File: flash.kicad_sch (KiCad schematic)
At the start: 1 part, among them U8 28F400

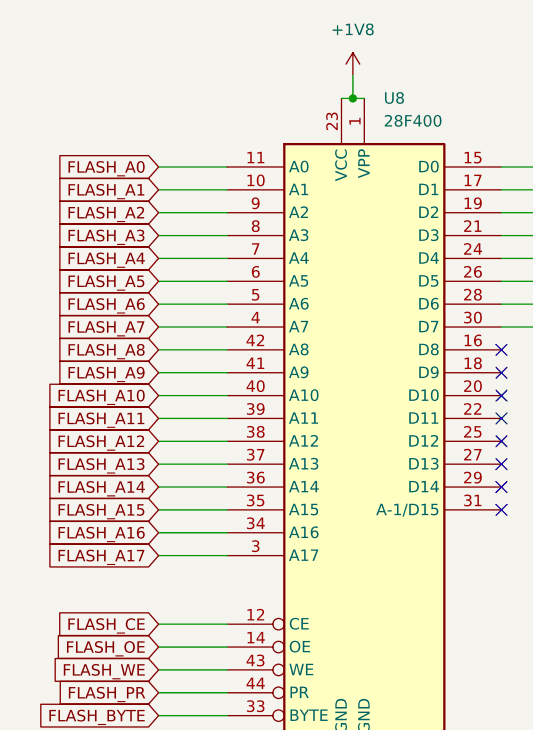
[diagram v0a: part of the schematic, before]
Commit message: morning
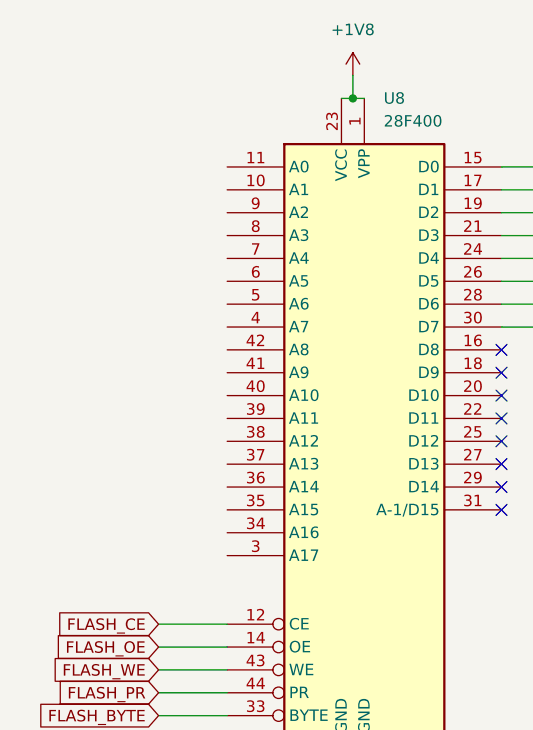
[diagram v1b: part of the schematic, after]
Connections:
- net FLASH_A0: no longer names the net of U8.11 (A0)
- net FLASH_A1: no longer names the net of U8.10 (A1)
- net FLASH_A10: no longer names the net of U8.40 (A10)
- net FLASH_A11: no longer names the net of U8.39 (A11)
- net FLASH_A12: no longer names the net of U8.38 (A12)
- net FLASH_A13: no longer names the net of U8.37 (A13)
- net FLASH_A14: no longer names the net of U8.36 (A14)
- net FLASH_A15: no longer names the net of U8.35 (A15)
- net FLASH_A16: no longer names the net of U8.34 (A16)
- net FLASH_A17: no longer names the net of U8.3 (A17)
- net FLASH_A2: no longer names the net of U8.9 (A2)
- net FLASH_A3: no longer names the net of U8.8 (A3)
- net FLASH_A4: no longer names the net of U8.7 (A4)
- net FLASH_A5: no longer names the net of U8.6 (A5)
- net FLASH_A6: no longer names the net of U8.5 (A6)
- net FLASH_A7: no longer names the net of U8.4 (A7)
- net FLASH_A8: no longer names the net of U8.42 (A8)
- net FLASH_A9: no longer names the net of U8.41 (A9)

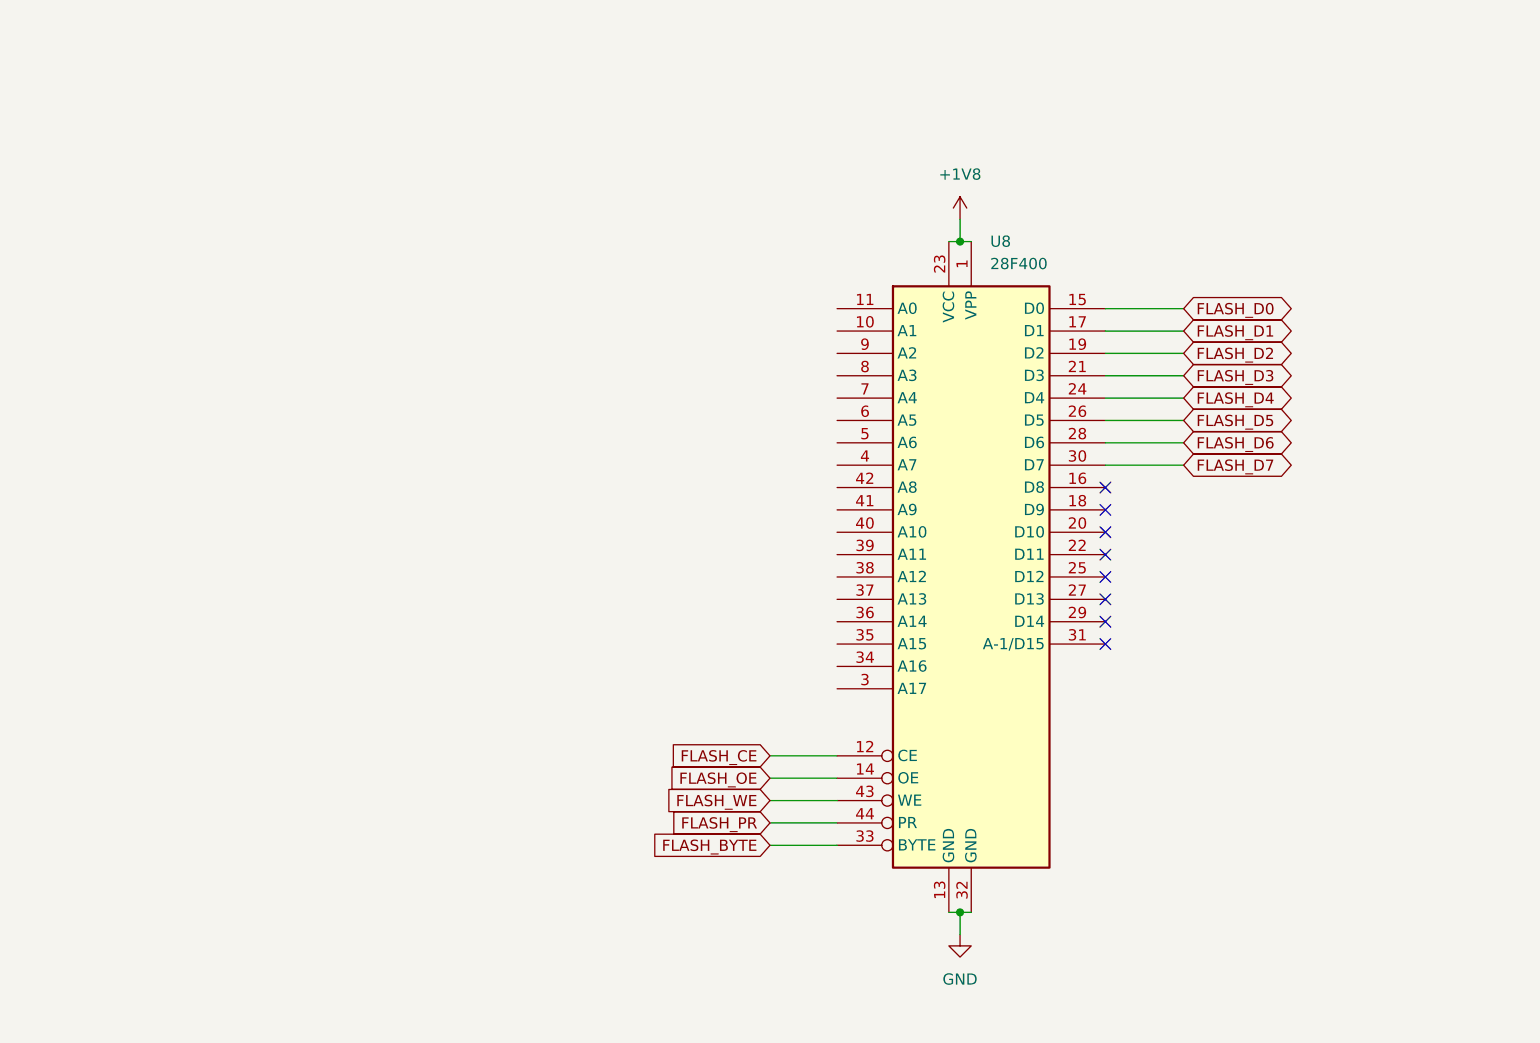
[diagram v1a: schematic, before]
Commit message: before caleb
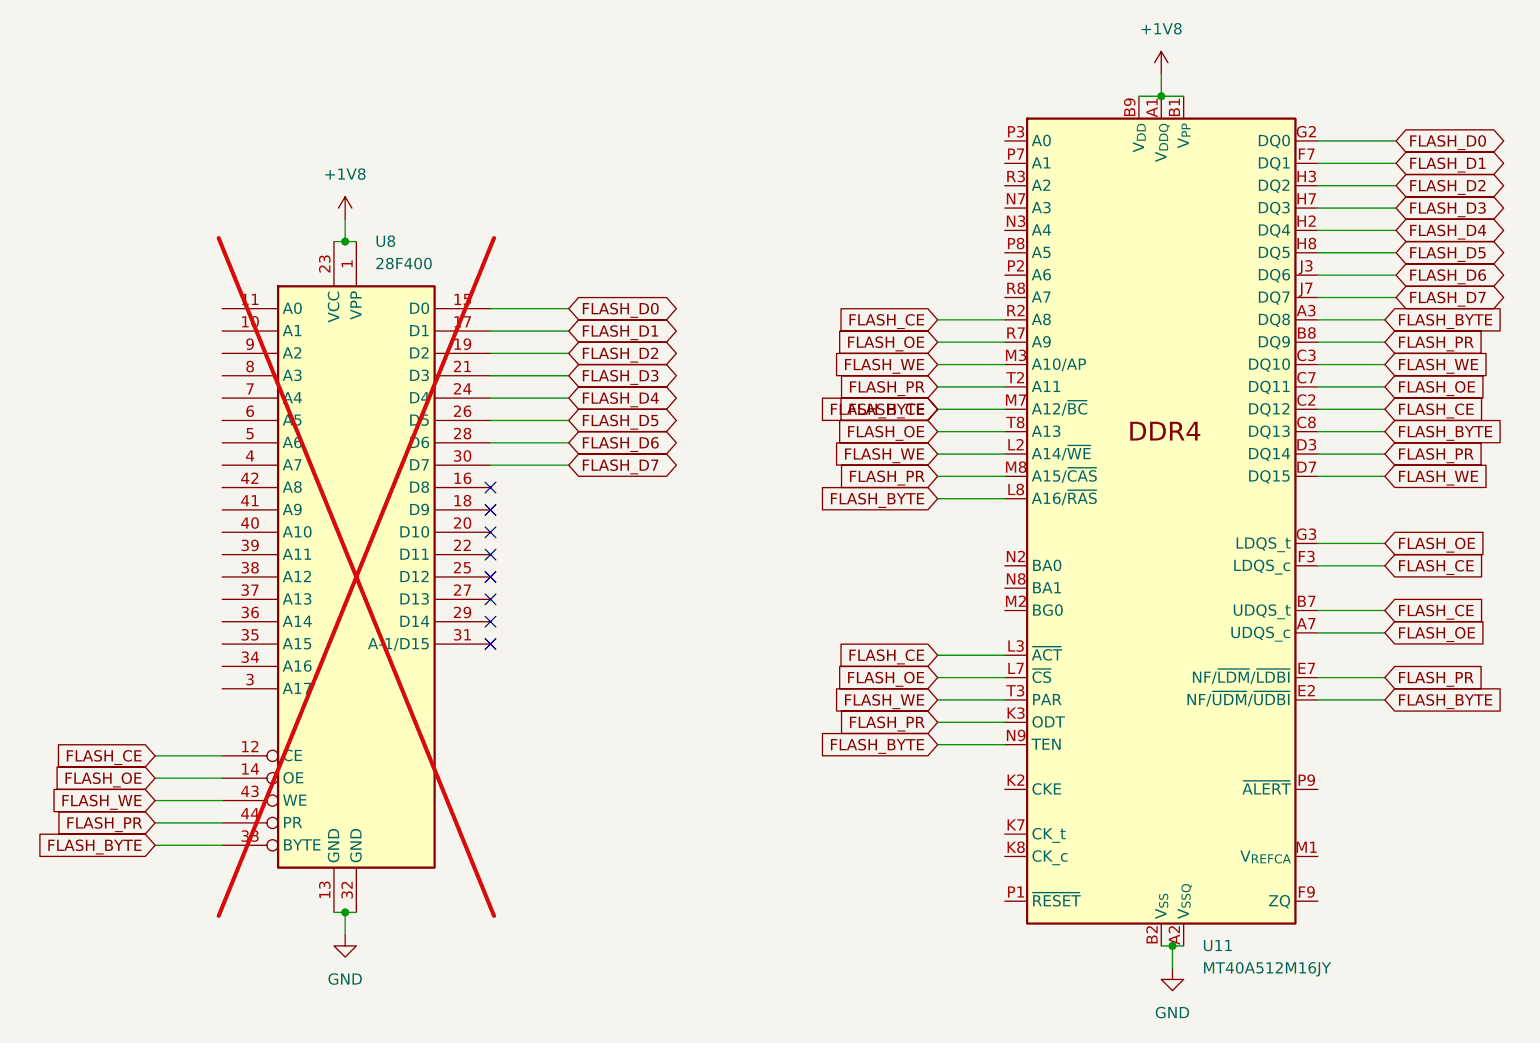
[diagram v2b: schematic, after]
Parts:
- added U11: MT40A512M16JY, Package_BGA:BGA-63_9x11mm_Layout10x12_P0.8mm, symbol Memory_RAM:MT40A512M16JY
- U8: now not fitted; now left out of the parts list
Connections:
- net FLASH_CE is gone; now on net FLASH_BYTE: U8.12 (CE)
- net +1V8: now also U11.A1 (V_{DDQ}), U11.A9 (V_{DDQ}), U11.B1 (V_{PP}), U11.B3 (V_{DD}), U11.B9 (V_{DD}), U11.C1 (V_{DDQ}), U11.D1 (V_{DD}), U11.D9 (V_{DDQ}), U11.F2 (V_{DDQ}), U11.F8 (V_{DDQ}), U11.G1 (V_{DDQ}), U11.G7 (V_{DD}), U11.G9 (V_{DDQ}), U11.J1 (V_{DD}), U11.J2 (V_{DDQ}), U11.J8 (V_{DDQ}), U11.J9 (V_{DD}), U11.L1 (V_{DD}), U11.L9 (V_{DD}), U11.R1 (V_{DD}), U11.R9 (V_{PP}), U11.T9 (V_{DD})
- net FLASH_BYTE: now also U11.A3 (DQ8), U11.B7 (UDQS_t), U11.C2 (DQ12), U11.C8 (DQ13), U11.E2 (NF/~{UDM}/~{UDBI}), U11.F3 (LDQS_c), U11.L3 (~{ACT}), U11.L8 (A16/~{RAS}), U11.M7 (A12/~{BC}), U11.N9 (TEN), U11.R2 (A8)
- net FLASH_D0: now also U11.G2 (DQ0)
- net FLASH_D1: now also U11.F7 (DQ1)
- net FLASH_D2: now also U11.H3 (DQ2)
- net FLASH_D3: now also U11.H7 (DQ3)
- net FLASH_D4: now also U11.H2 (DQ4)
- net FLASH_D5: now also U11.H8 (DQ5)
- net FLASH_D6: now also U11.J3 (DQ6)
- net FLASH_D7: now also U11.J7 (DQ7)
- net FLASH_OE: now also U11.A7 (UDQS_c), U11.C7 (DQ11), U11.G3 (LDQS_t), U11.L7 (~{CS}), U11.R7 (A9), U11.T8 (A13)
- net FLASH_PR: now also U11.B8 (DQ9), U11.D3 (DQ14), U11.E7 (NF/~{LDM}/~{LDBI}), U11.K3 (ODT), U11.M8 (A15/~{CAS}), U11.T2 (A11)
- net FLASH_WE: now also U11.C3 (DQ10), U11.D7 (DQ15), U11.L2 (A14/~{WE}), U11.M3 (A10/AP), U11.T3 (PAR)
- net GND: now also U11.A2 (V_{SSQ}), U11.A8 (V_{SSQ}), U11.B2 (V_{SS}), U11.C9 (V_{SSQ}), U11.D2 (V_{SSQ}), U11.D8 (V_{SSQ}), U11.E1 (V_{SS}), U11.E3 (V_{SSQ}), U11.E8 (V_{SSQ}), U11.E9 (V_{SS}), U11.F1 (V_{SSQ}), U11.G8 (V_{SS}), U11.H1 (V_{SSQ}), U11.H9 (V_{SSQ}), U11.K1 (V_{SS}), U11.K9 (V_{SS}), U11.M9 (V_{SS}), U11.N1 (V_{SS}), U11.T1 (V_{SS})

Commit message: after rough draft submission
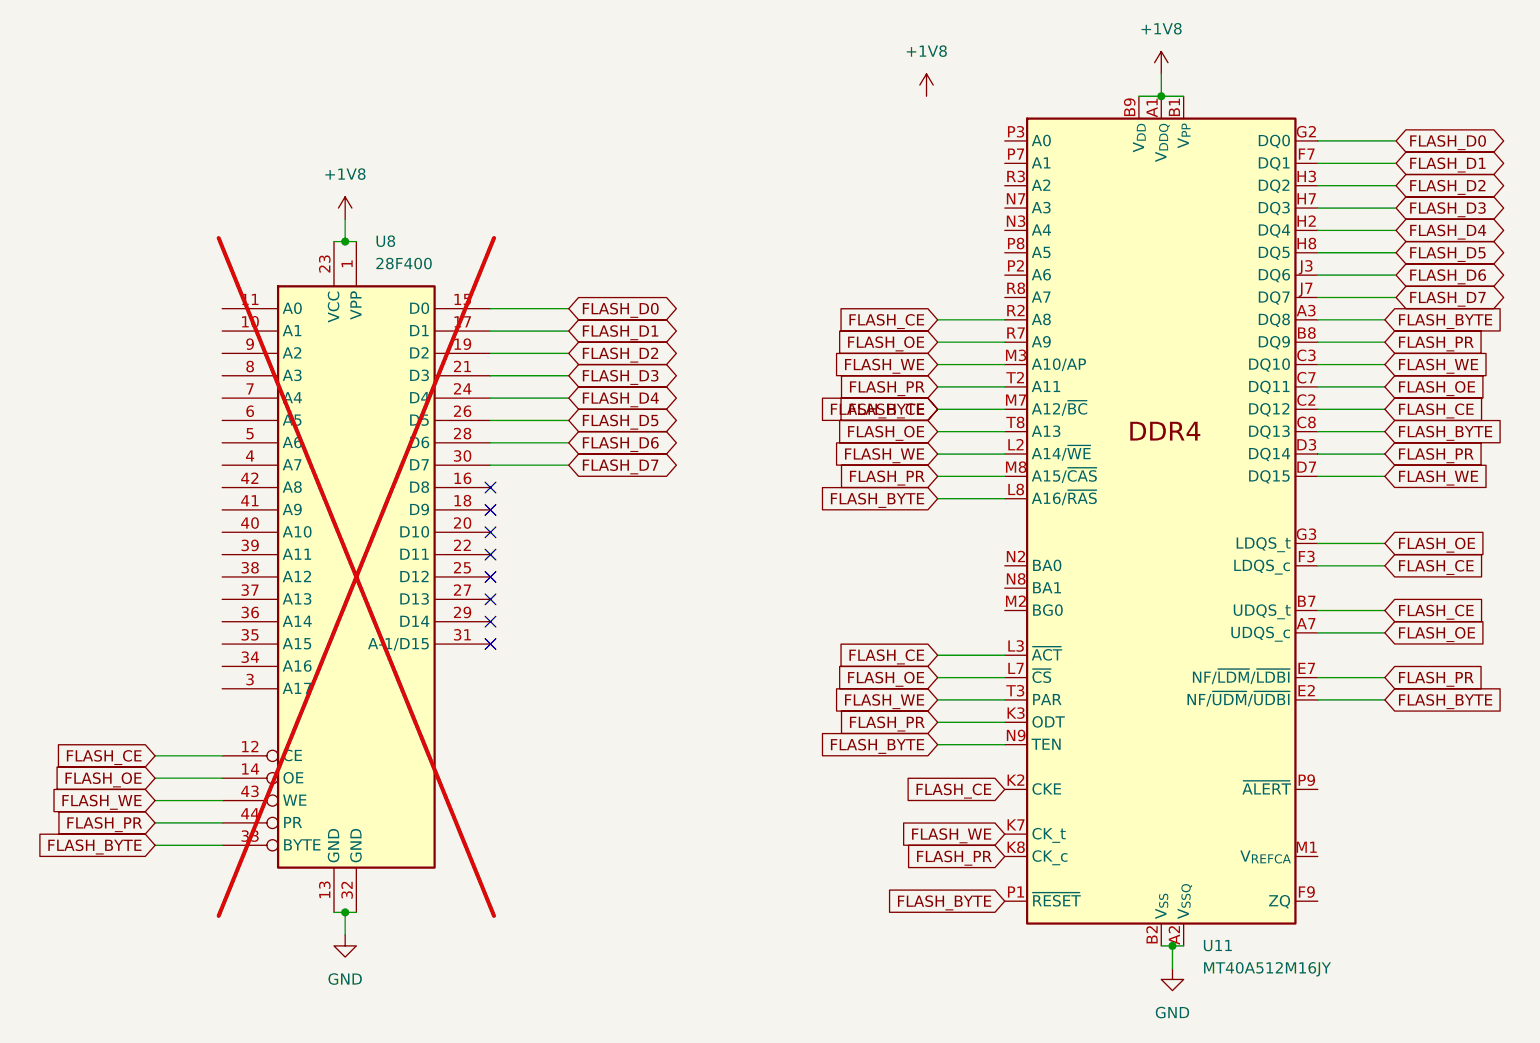
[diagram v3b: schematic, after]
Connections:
- net FLASH_BYTE: now also U11.K2 (CKE), U11.P1 (~{RESET})
- net FLASH_PR: now also U11.K8 (CK_c)
- net FLASH_WE: now also U11.K7 (CK_t)
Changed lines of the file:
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@@
+		)
+	)
+	(global_label "FLASH_WE"
+		(shape input)
+		(at 162.56 130.81 180)
+		(effects
+			(font
+				(size 1.27 1.27)
+			)
+			(justify right)
+		)
+		(property "Intersheetrefs" "${INTERSHEET_REFS}"
+			(at 162.56 130.81 0)
+			(effects
+				(font
+					(size 1.27 1.27)
+				)
+				(hide yes)
+			)
 		)
 	)
@@
 		(property "Intersheetrefs" "${INTERSHEET_REFS}"
 			(at 66.04 124.46 0)
+			(effects
+				(font
+					(size 1.27 1.27)
+				)
+				(hide yes)
+			)
+		)
+	)
+	(global_label "FLASH_PR"
+		(shape input)
+		(at 162.56 133.35 180)
+		(effects
+			(font
+				(size 1.27 1.27)
+			)
+			(justify right)
+		)
+		(property "Intersheetrefs" "${INTERSHEET_REFS}"
+			(at 162.56 133.35 0)
 			(effects
 				(font
@@
 	(global_label "FLASH_CE"
 		(shape input)
+		(at 162.56 125.73 180)
+		(effects
+			(font
+				(size 1.27 1.27)
+			)
+			(justify right)
+		)
+		(property "Intersheetrefs" "${INTERSHEET_REFS}"
+			(at 162.56 125.73 0)
+			(effects
+				(font
+					(size 1.27 1.27)
+				)
+				(hide yes)
+			)
+		)
+	)
+	(global_label "FLASH_CE"
+		(shape input)
 		(at 205.74 82.55 0)
 		(effects
@@
 		(property "Intersheetrefs" "${INTERSHEET_REFS}"
 			(at 205.74 107.95 0)
+			(effects
+				(font
+					(size 1.27 1.27)
+				)
+				(hide yes)
+			)
+		)
+	)
+	(global_label "FLASH_BYTE"
+		(shape input)
+		(at 162.56 138.43 180)
+		(effects
+			(font
+				(size 1.27 1.27)
+			)
+			(justify right)
+		)
+		(property "Intersheetrefs" "${INTERSHEET_REFS}"
+			(at 162.56 138.43 0)
 			(effects
 				(font
@@
 					(unit 1)
 				)
+			)
+		)
+	)
+	(symbol
+		(lib_id "power:+1V8")
+		(at 153.67 46.99 0)
+		(unit 1)
+		(exclude_from_sim no)
+		(in_bom yes)
+		(on_board yes)
+		(dnp no)
+		(fields_autoplaced yes)
+		(property "Reference" "#PWR054"
+			(at 153.67 50.8 0)
+			(effects
+				(font
+					(size 1.27 1.27)
+				)
+				(hide yes)
+			)
+		)
+		(property "Value" "+1V8"
+			(at 153.67 41.91 0)
+			(effects
+				(font
+					(size 1.27 1.27)
+				)
+			)
+		)
+		(property "Footprint" ""
+			(at 153.67 46.99 0)
+			(effects
+				(font
+					(size 1.27 1.27)
+				)
+				(hide yes)
+			)
+		)
+		(property "Datasheet" ""
+			(at 153.67 46.99 0)
+			(effects
+				(font
+					(size 1.27 1.27)
+				)
+				(hide yes)
+			)
+		)
+		(property "Description" "Power symbol creates a global label with name \"+1V8\""
+			(at 153.67 46.99 0)
+			(effects
+				(font
+					(size 1.27 1.27)
+				)
+				(hide yes)
+			)
+		)
+		(pin "1"
+		)
+		(instances
+			(project "spacex-sbc"
+				(path "/2cb83ae2-abb4-4908-af16-d6e3533577eb/f0f01e93-37ca-4d9b-b962-624941e092bb"
+					(reference "#PWR054")
+					(unit 1)
+				)
